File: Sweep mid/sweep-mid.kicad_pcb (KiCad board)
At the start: 2 copper layers, 229.5 x 95.2 mm, 63 parts, among them J1 AudioJack4dpb, J2 AudioJack4dpb, SW10 SW_Push, SW11 SW_Push, SW11_r1 SW_Push, SW12 SW_Push, SW12_r1 SW_Push, SW13_r1 SW_Push, SW14 SW_Push, SW15 SW_Push, SW15_r1 SW_Push, SW16 SW_Push, SW16_r1 SW_Push, SW17 SW_Push, SW17_r1 SW_Push, SW18 SW_Push, SW18_r1 SW_Push, SW2 SW_Push, SW2 SW_SPDT, SW20 SW_Push, SW20_r1 SW_Push, SW21 SW_Push, SW21_r1 SW_Push, SW2_r1 SW_Push, SW3 SW_Push, SW3_r1 SW_Push, SW4 SW_Push, SW4_r1 SW_Push, SW5 SW_Push, SW5_r1 SW_Push, SW6 SW_Push, SW6_r1 SW_Push, SW7_r1 SW_Push, SW8 SW_Push, SW8_r1 SW_Push, SW9 SW_Push, SW9_r1 SW_Push, U1 ProMicro-kbd, U2 ProMicro-kbd

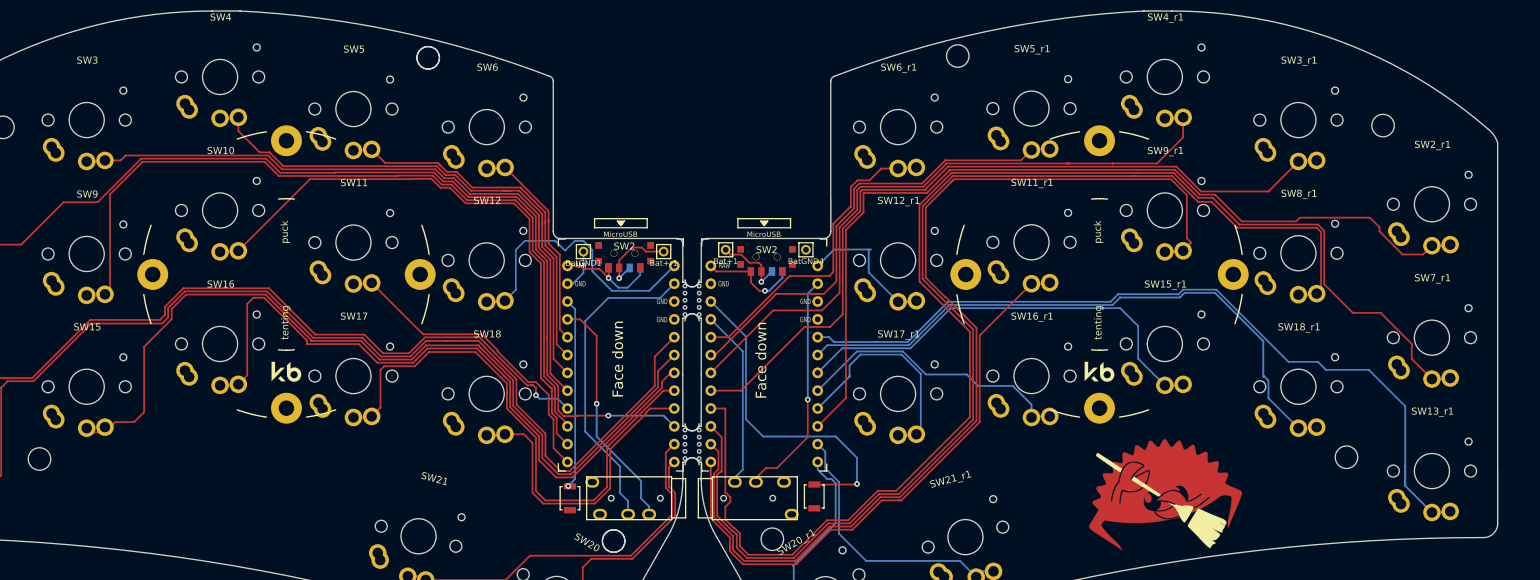
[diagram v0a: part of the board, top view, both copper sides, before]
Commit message: Add files via upload
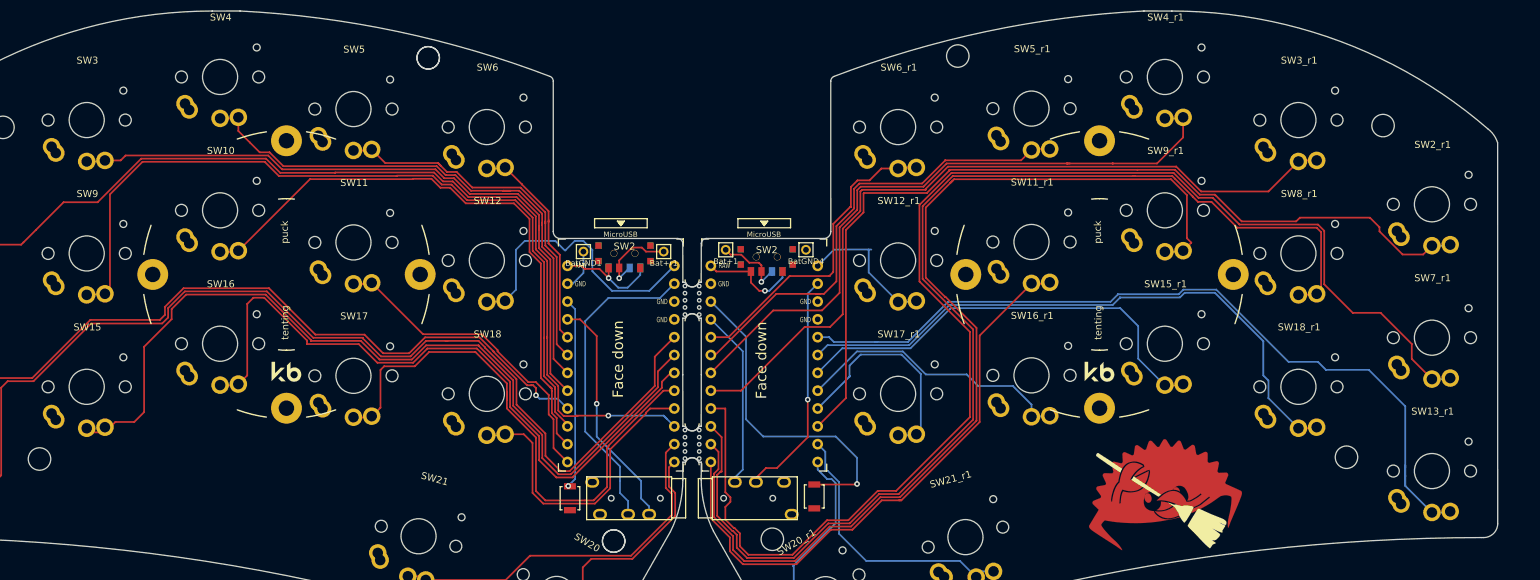
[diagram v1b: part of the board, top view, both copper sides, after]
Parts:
- moved SW16_r1 0.10 mm to (198.6, 101.4)
- moved SW9 0.07 mm to (64.0, 84.0)
- moved SW11_r1 0.05 mm to (198.6, 82.4)
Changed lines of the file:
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@@
   )
   (footprint "sadik:gateron-ks27-choc-v1" (layer "F.Cu")
-    (at 101.994 63.432)
+    (at 102 63.432)
     (attr through_hole)
     (fp_text reference "SW5" (at 0.1 -8.5 unlocked) (layer "F.SilkS")
@@
   )
   (footprint "sadik:gateron-ks27-choc-v1" (layer "F.Cu")
-    (at 64 84.074)
+    (at 64 84)
     (attr through_hole)
     (fp_text reference "SW9" (at 0.1 -8.5 unlocked) (layer "F.SilkS")
@@
   )
   (footprint "sadik:gateron-ks27-choc-v1" (layer "F.Cu")
-    (at 83 77.878)
+    (at 83 77.86)
     (attr through_hole)
     (fp_text reference "SW10" (at 0.1 -8.5 unlocked) (layer "F.SilkS")
@@
   )
   (footprint "sadik:gateron-ks27-choc-v1" (layer "F.Cu")
-    (at 102 82.45)
+    (at 102 82.432)
     (attr through_hole)
     (fp_text reference "SW11" (at 0.1 -8.5 unlocked) (layer "F.SilkS")
@@
   )
   (footprint "sadik:gateron-ks27-choc-v1" (layer "F.Cu")
-    (at 120.98 84.99)
+    (at 121 85)
     (attr through_hole)
     (fp_text reference "SW12" (at 0.1 -8.5 unlocked) (layer "F.SilkS")
@@
   )
   (footprint "sadik:gateron-ks27-choc-v1" (layer "F.Cu")
-    (at 64 102.992)
+    (at 64 103)
     (attr through_hole)
     (fp_text reference "SW15" (at 0.1 -8.5 unlocked) (layer "F.SilkS")
@@
   )
   (footprint "sadik:gateron-ks27-choc-v1" (layer "F.Cu")
-    (at 83 96.896)
+    (at 83 96.86)
     (attr through_hole)
     (fp_text reference "SW16" (at 0.1 -8.5 unlocked) (layer "F.SilkS")
@@
   )
   (footprint "sadik:gateron-ks27-choc-v1" (layer "F.Cu")
-    (at 102 101.468)
+    (at 102 101.432)
     (attr through_hole)
     (fp_text reference "SW17" (at 0.1 -8.5 unlocked) (layer "F.SilkS")
@@
   )
   (footprint "sadik:gateron-ks27-choc-v1" (layer "F.Cu")
-    (at 120.98 104.008)
+    (at 121 104)
     (attr through_hole)
     (fp_text reference "SW18" (at 0.1 -8.5 unlocked) (layer "F.SilkS")
@@
   )
   (footprint "sadik:gateron-ks27-choc-v1" (layer "F.Cu")
-    (at 198.58584 82.418)
+    (at 198.58584 82.368)
     (attr through_hole)
     (fp_text reference "SW11_r1" (at 0.1 -8.5 unlocked) (layer "F.SilkS")
@@
   )
   (footprint "sadik:gateron-ks27-choc-v1" (layer "F.Cu")
-    (at 217.58784 96.896)
+    (at 217.58584 96.86)
     (attr through_hole)
     (fp_text reference "SW15_r1" (at 0.1 -8.5 unlocked) (layer "F.SilkS")
@@
   )
   (footprint "sadik:gateron-ks27-choc-v1" (layer "F.Cu")
-    (at 198.58584 101.468)
+    (at 198.58584 101.368)
     (attr through_hole)
     (fp_text reference "SW16_r1" (at 0.1 -8.5 unlocked) (layer "F.SilkS")
@@
   )
   (footprint "sadik:gateron-ks27-choc-v1" (layer "F.Cu")
-    (at 236.61384 83.974)
+    (at 236.61384 84)
     (attr through_hole)
     (fp_text reference "SW8_r1" (at 0.1 -8.5 unlocked) (layer "F.SilkS")
@@
   )
   (footprint "sadik:gateron-ks27-choc-v1" (layer "F.Cu")
-    (at 217.58784 77.878)
+    (at 217.58784 77.86)
     (attr through_hole)
     (fp_text reference "SW9_r1" (at 0.1 -8.5 unlocked) (layer "F.SilkS")
@@
   )
   (footprint "sadik:gateron-ks27-choc-v1" (layer "F.Cu")
-    (at 236.61384 102.992)
+    (at 236.61384 103)
     (attr through_hole)
     (fp_text reference "SW18_r1" (at 0.1 -8.5 unlocked) (layer "F.SilkS")
@@
   )
   (footprint "sadik:gateron-ks27-choc-v1" (layer "F.Cu")
-    (at 179.58584 84.99)
+    (at 179.58584 85)
     (attr through_hole)
     (fp_text reference "SW12_r1" (at 0.1 -8.5 unlocked) (layer "F.SilkS")
@@
   )
   (footprint "sadik:gateron-ks27-choc-v1" (layer "F.Cu")
-    (at 179.58584 104.008)
+    (at 179.58584 104)
     (attr through_hole)
     (fp_text reference "SW17_r1" (at 0.1 -8.5 unlocked) (layer "F.SilkS")
@@
   (gr_arc (start 170.429595 58.79247) (mid 192.154196 52.385453) (end 214.614613 49.463504) (layer "Edge.Cuts") (width 0.05))
   (gr_line (start 262.68984 124.474571) (end 262.964838 124.473917) (layer "Edge.Cuts") (width 0.05))
-  (gr_arc (start 264.999839 122.542999) (mid 264.377307 123.924717) (end 262.964838 124.473917) (layer "Edge.Cuts") (width 0.05))
+  (gr_arc (start 264.999839 122.542999) (mid 264.377307 123.924716) (end 262.964838 124.473917) (layer "Edge.Cuts") (width 0.05))
   (gr_arc (start 169.99484 59.473) (mid 170.112806 59.069226) (end 170.429595 58.79247) (layer "Edge.Cuts") (width 0.05))
   (gr_line (start 151.53384 88.11) (end 151.1935 88.11) (layer "Edge.Cuts") (width 0.05))
@@
   (segment (start 211.168092 90.329908) (end 210.15744 91.34056) (width 0.25) (layer "B.Cu") (net 30))
   (segment (start 211.168092 90.264092) (end 219.743626 90.264092) (width 0.25) (layer "B.Cu") (net 30))
-  (segment (start 231.61384 101.38016) (end 231.61384 101.63416) (width 0.25) (layer "B.Cu") (net 30))
   (segment (start 231.61384 101.38016) (end 232.339261 102.105581) (width 0.25) (layer "B.Cu") (net 30))
   (segment (start 186.88518 91.34056) (end 186.86487 91.36087) (width 0.25) (layer "B.Cu") (net 30))

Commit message: thumb nudge
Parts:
- removed SW20_r1, SW21_r1: SW_Push, sadik:gateron-ks27-choc-v1
- added SW20-r: SW_Push, kbd:gateron-ks27-choc-v1, B.Cu at (169.3, 132.5)
- added SW21: SW_Push, kbd:gateron-ks27-choc-v1, B.Cu at (189.0, 124.3)
- SW20, SW21: footprint sadik:gateron-ks27-choc-v1 -> kbd:gateron-ks27-choc-v1
- moved SW21 0.06 mm to (111.2, 124.3)
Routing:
- net Switch16_r: track 39.2 -> 37.8 mm
- net gnd: track 11.3 -> 10.2 mm
